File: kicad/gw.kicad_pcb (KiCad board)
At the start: 2 copper layers, 21 parts, among them IC1 ATMEGA8A-A, P1 12v-gnd-clunet, P2 CONN_01X08, P3 CONN_RST, P9 CON_RPI_1-10, Q1 BC847, Q2 BC847, U1 MC78L05ACD

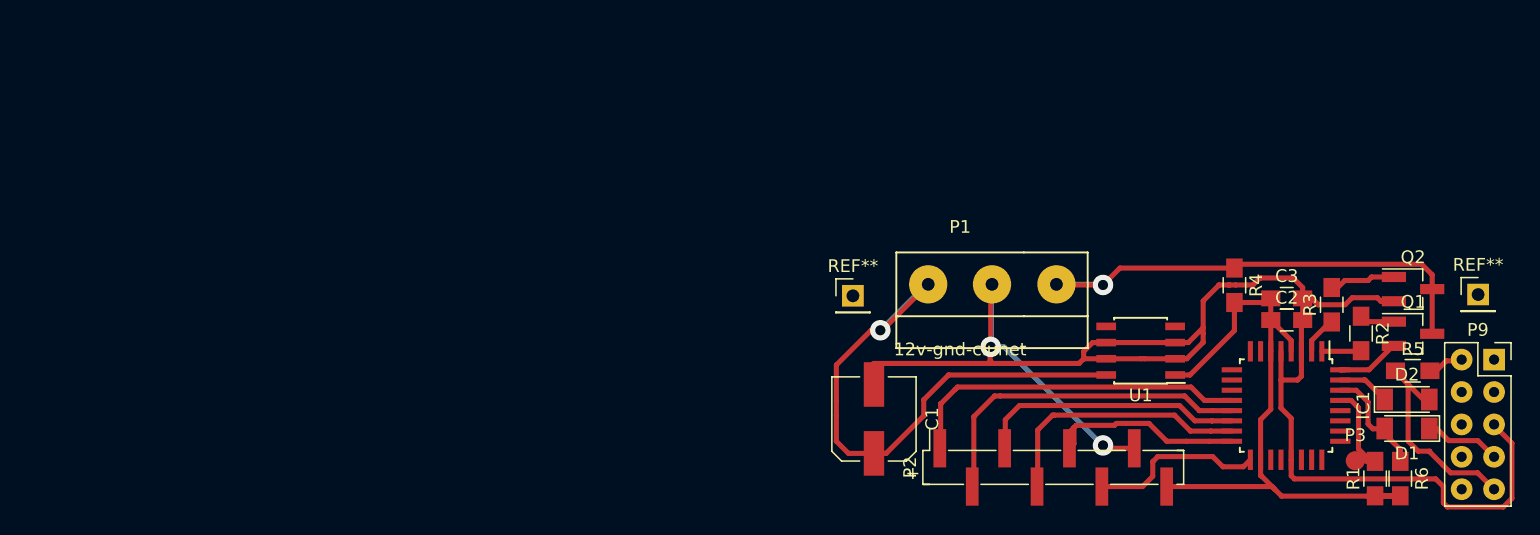
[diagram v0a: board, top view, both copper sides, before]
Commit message: ЧТо-то еще поменялось
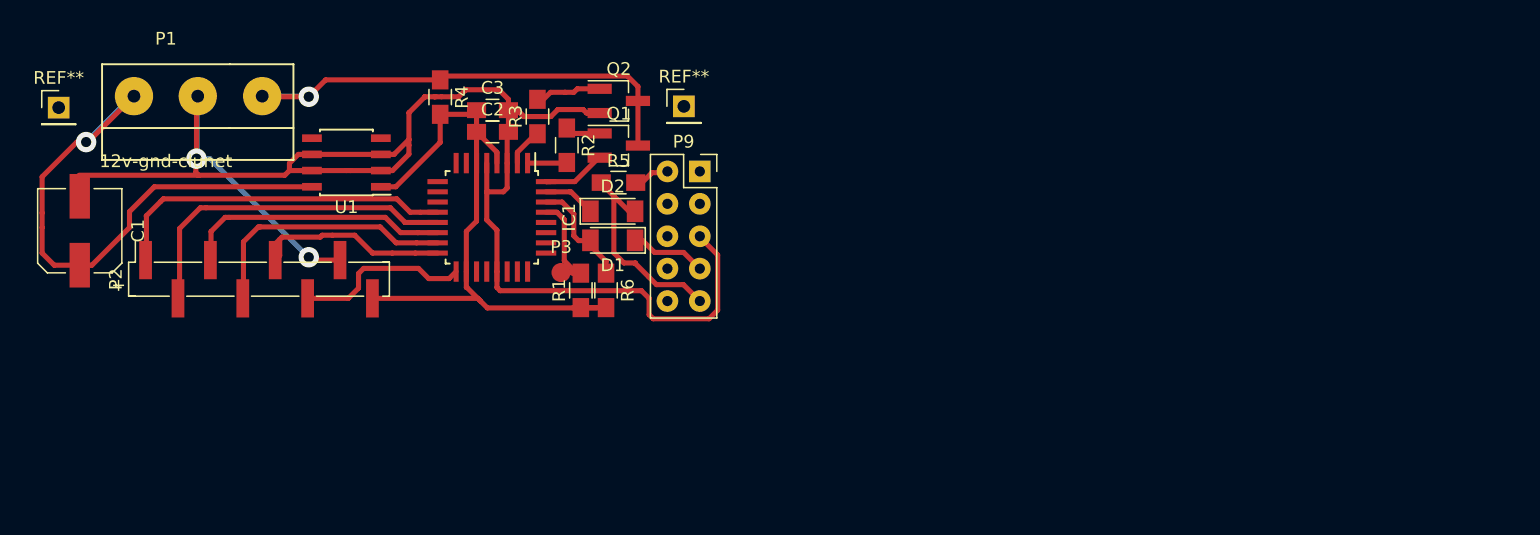
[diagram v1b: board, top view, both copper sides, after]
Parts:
- moved IC1 64.0 mm to (55.4, 32.0)
- moved P2 64.0 mm to (37.1, 36.9)
- moved R2 64.0 mm to (61.3, 26.4)
- moved C2 64.0 mm to (55.5, 25.4)
- moved C3 64.0 mm to (55.5, 23.6)
- moved D1 64.0 mm to (64.9, 33.9)
- moved D2 64.0 mm to (64.9, 31.6)
- moved P3 64.0 mm to (60.8, 36.4)
- moved Q1 64.0 mm to (65.3, 26.4)
- moved Q2 64.0 mm to (65.3, 22.9)
- moved R1 64.0 mm to (62.4, 37.8)
- moved R5 64.0 mm to (65.3, 29.3)
- moved R6 64.0 mm to (64.3, 37.8)
- moved REF** 64.0 mm to (21.4, 23.4)
- moved U1 64.0 mm to (44.0, 27.8)
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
